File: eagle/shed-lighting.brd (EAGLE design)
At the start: 98.7 x 68.6 mm, 25 parts, among them X1 22-23-2021, X2 22-23-2021, X3 22-23-2021

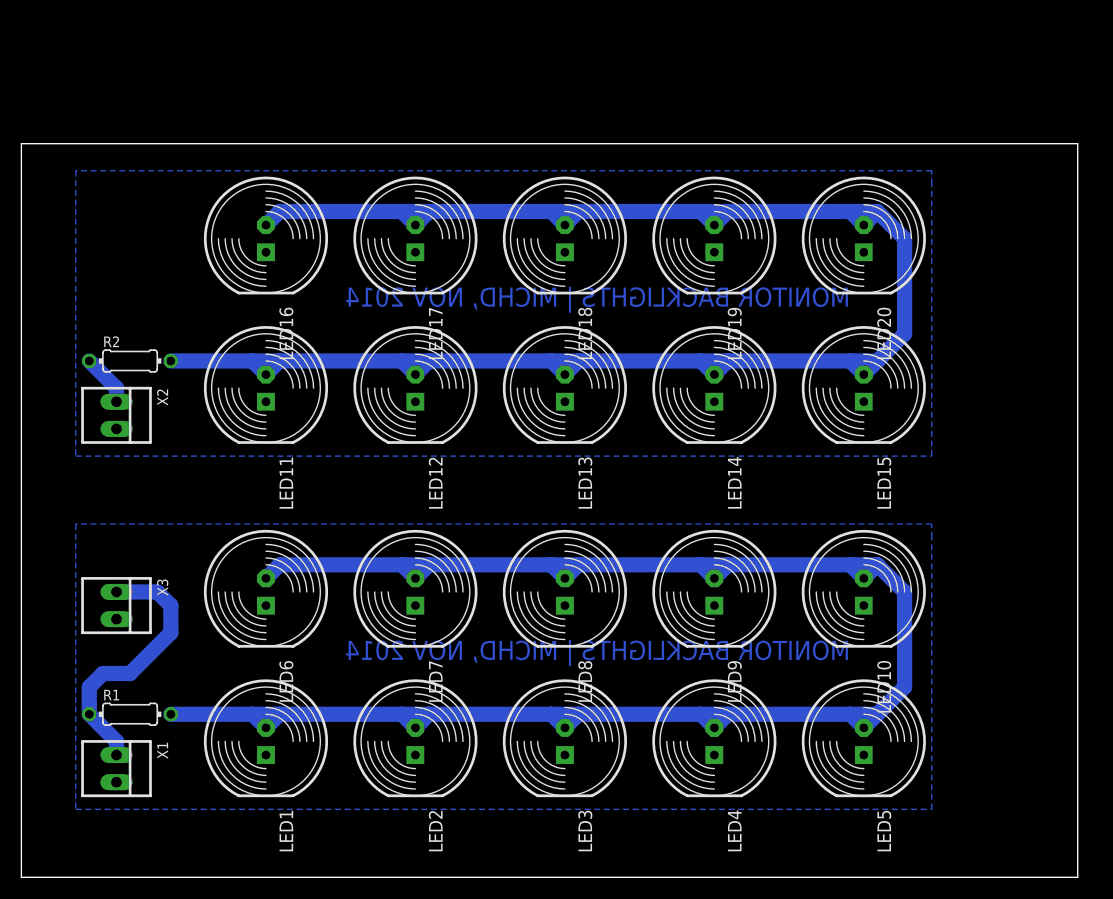
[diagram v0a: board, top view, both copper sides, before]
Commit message: Design schematic and board
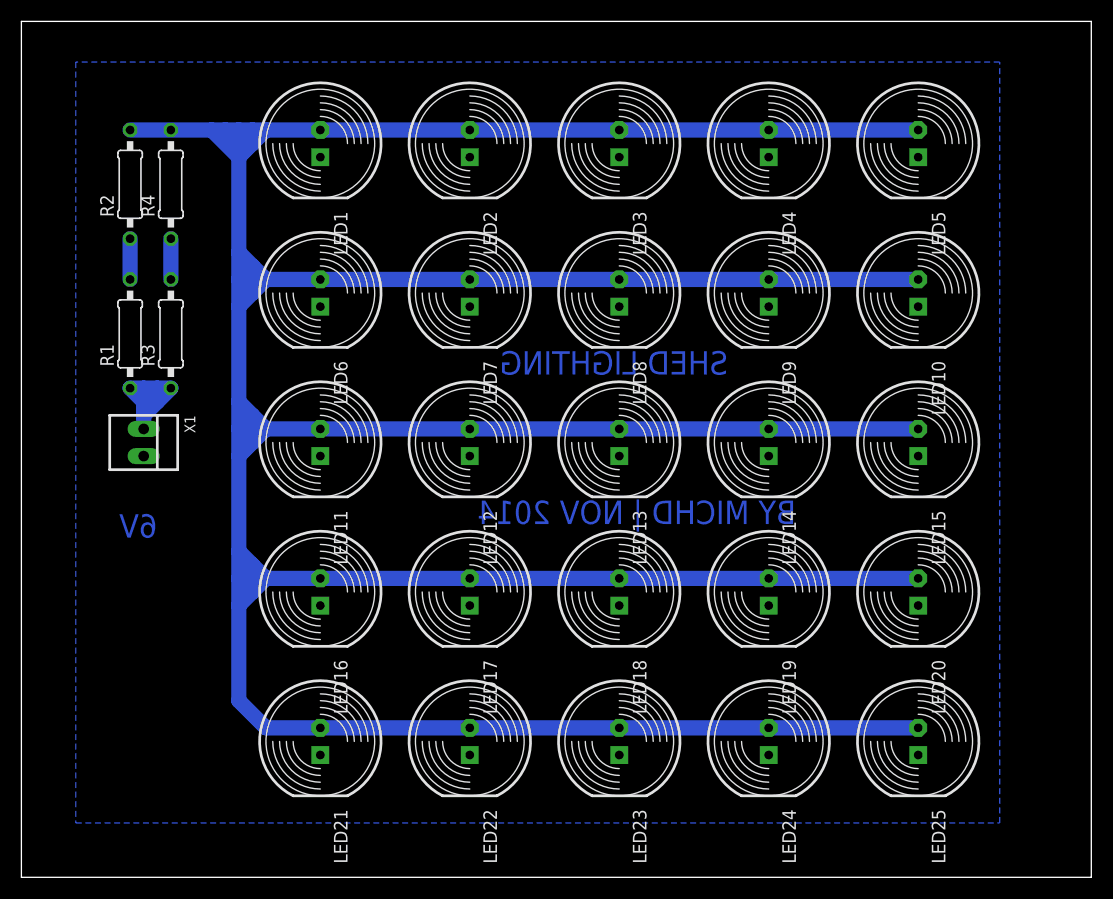
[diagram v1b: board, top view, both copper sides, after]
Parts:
- removed X2, X3: 22-23-2021, con-molex:22-23-2021
- added LED21, LED22, LED23, LED24, LED25: (no value), led:LED10MM
- added R3, R4: 10R, rcl:0207/10
- R1, R2: value 8R2 -> 10R; device rcl:0204/7 -> rcl:0207/10
- moved LED1 56.1 mm to (27.9, 68.6)
- moved LED2 56.1 mm to (41.9, 68.6)
- moved LED3 56.1 mm to (55.9, 68.6)
- moved LED4 56.1 mm to (69.8, 68.6)
- moved LED5 56.1 mm to (83.8, 68.6)
- moved R1 35.6 mm to (10.2, 50.8), turned to 90 degrees
- moved LED16 33.4 mm to (27.9, 26.7)
- moved LED18 33.4 mm to (55.9, 26.7)
- moved LED17 33.4 mm to (41.9, 26.7)
- moved LED19 33.4 mm to (69.8, 26.7)
- moved LED20 33.4 mm to (83.8, 26.7)
- moved X1 30.6 mm to (11.4, 40.6)
- moved LED6 28.4 mm to (27.9, 54.6)
- moved LED8 28.4 mm to (55.9, 54.6)
- moved LED10 28.4 mm to (83.8, 54.6)
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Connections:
- net GND: now also LED21.K, LED22.K, LED23.K, LED24.K, LED25.K; no longer X2.2, X3.2
- net N$1: now also R2.1; no longer LED1.A, LED10.A, LED2.A, LED3.A, LED4.A, LED5.A, LED6.A, LED7.A, LED8.A, LED9.A
- net N$2: now also R3.2, R4.1; no longer LED11.A, LED12.A, LED13.A, LED14.A, LED15.A, LED16.A, LED17.A, LED18.A, LED19.A, LED20.A, R2.2
- net N$4: now also LED1.A, LED10.A, LED11.A, LED12.A, LED13.A, LED14.A, LED15.A, LED16.A, LED17.A, LED18.A, LED19.A, LED2.A, LED20.A, LED21.A, LED22.A, LED23.A, LED24.A, LED25.A, LED3.A, LED4.A, LED5.A, LED6.A, LED7.A, LED8.A, LED9.A, R2.2, R4.2; no longer R2.1, X2.1
- net N$5: now also R3.1; no longer X3.1
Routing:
- net N$4: track 4.86 -> 427.2 mm
- net N$1: track 172.1 -> 3.81 mm
- net N$2: track 172.1 -> 3.81 mm
- net N$5: track 25.3 -> 14.3 mm
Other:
- board size 98.7 x 68.6 mm -> 100 x 80 mm
- board text added: "6V"
- board text added: "BY MICHD | NOV 2014"
- board text added: "SHED LIGHTING"
- board text removed: "MONITOR BACKLIGHTS | MICHD, NOV 2014"
